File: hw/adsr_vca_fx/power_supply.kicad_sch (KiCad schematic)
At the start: 6 parts, among them J1 Conn_01x03, J2 Conn_02x02_Odd_Even, J3 Conn_02x02_Odd_Even, U1 TL972

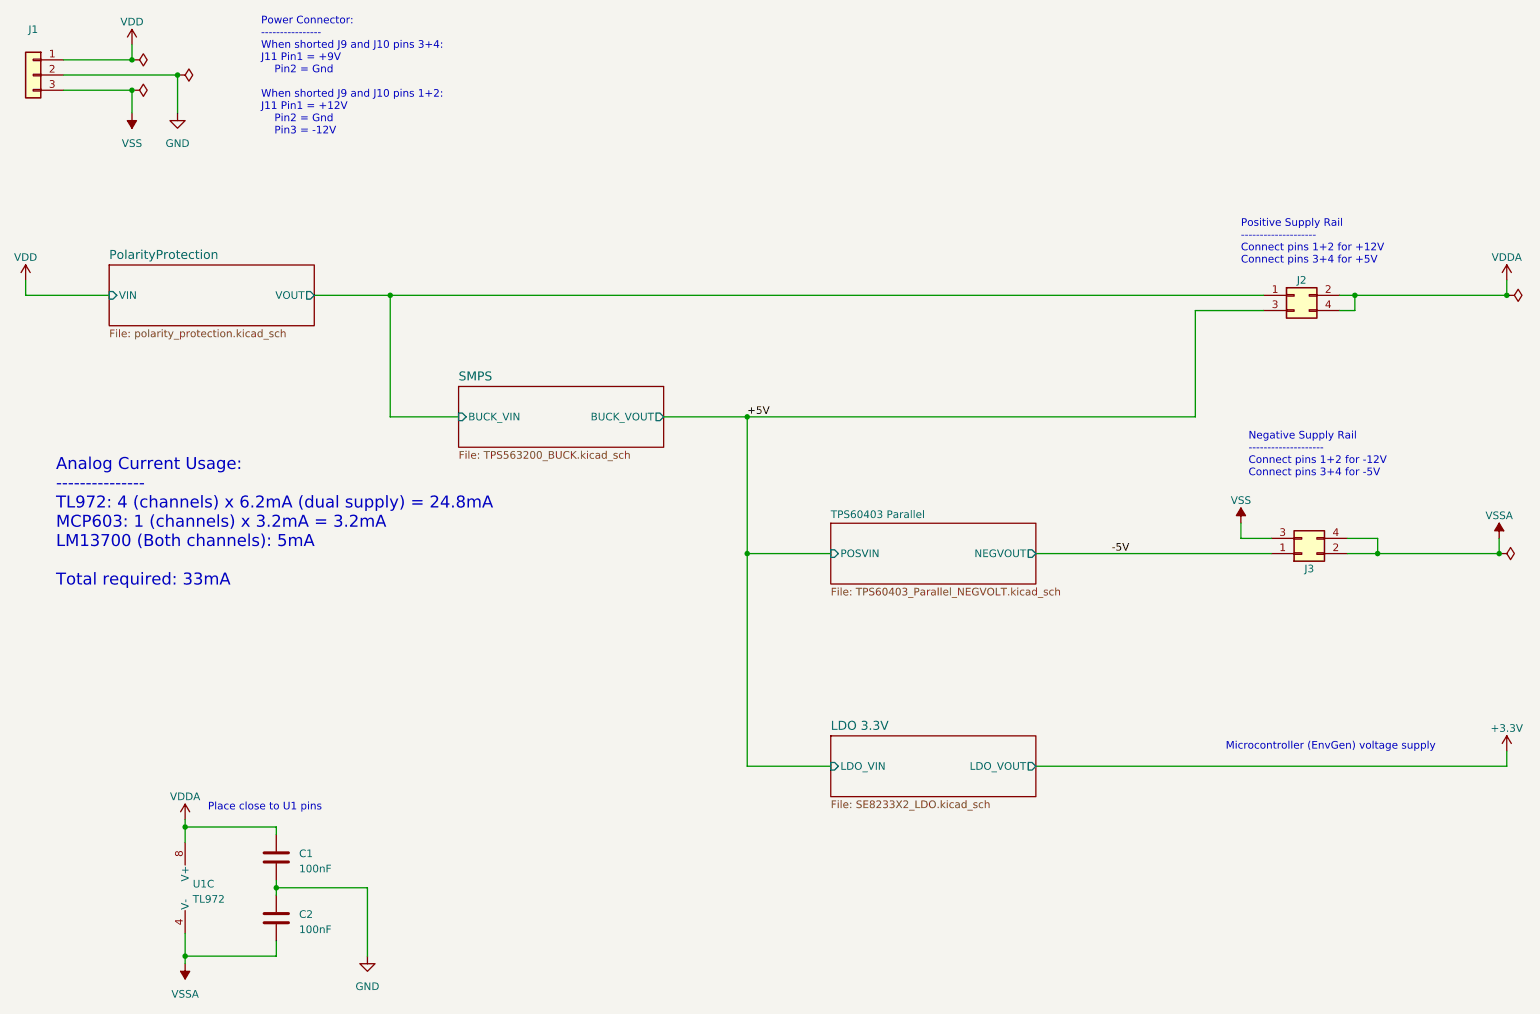
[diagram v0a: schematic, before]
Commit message: completed layout
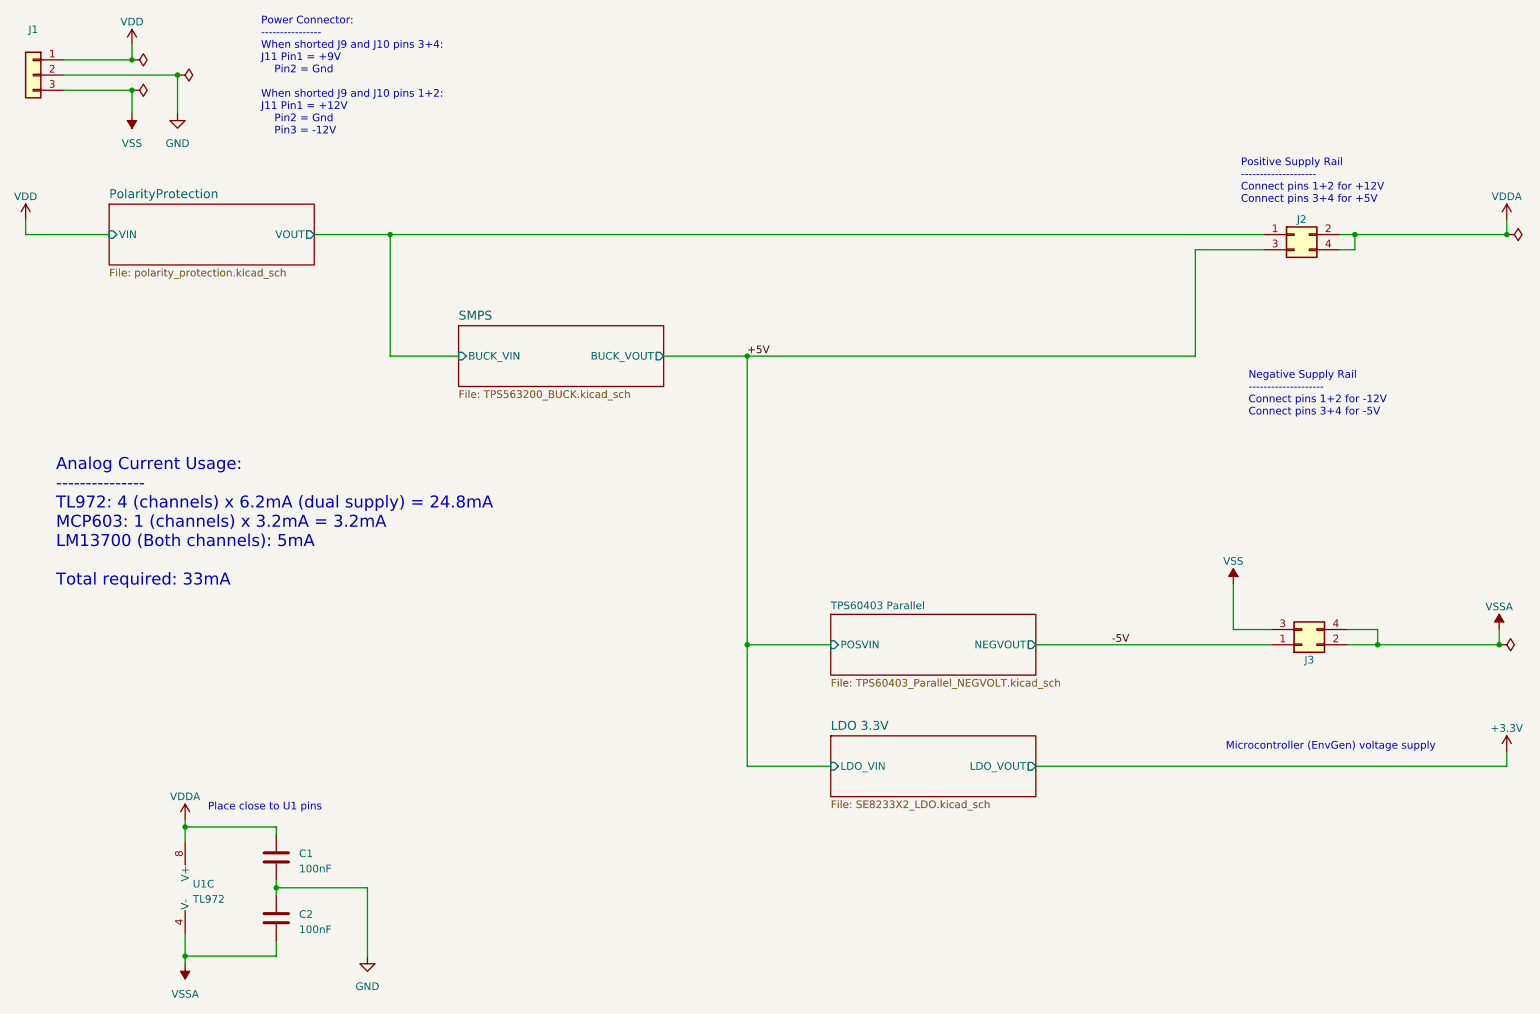
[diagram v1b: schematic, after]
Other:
- moved on the sheet: J2, J3
